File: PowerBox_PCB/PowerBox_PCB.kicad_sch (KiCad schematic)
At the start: 24 parts, among them SW1 SW_DPDT_x2

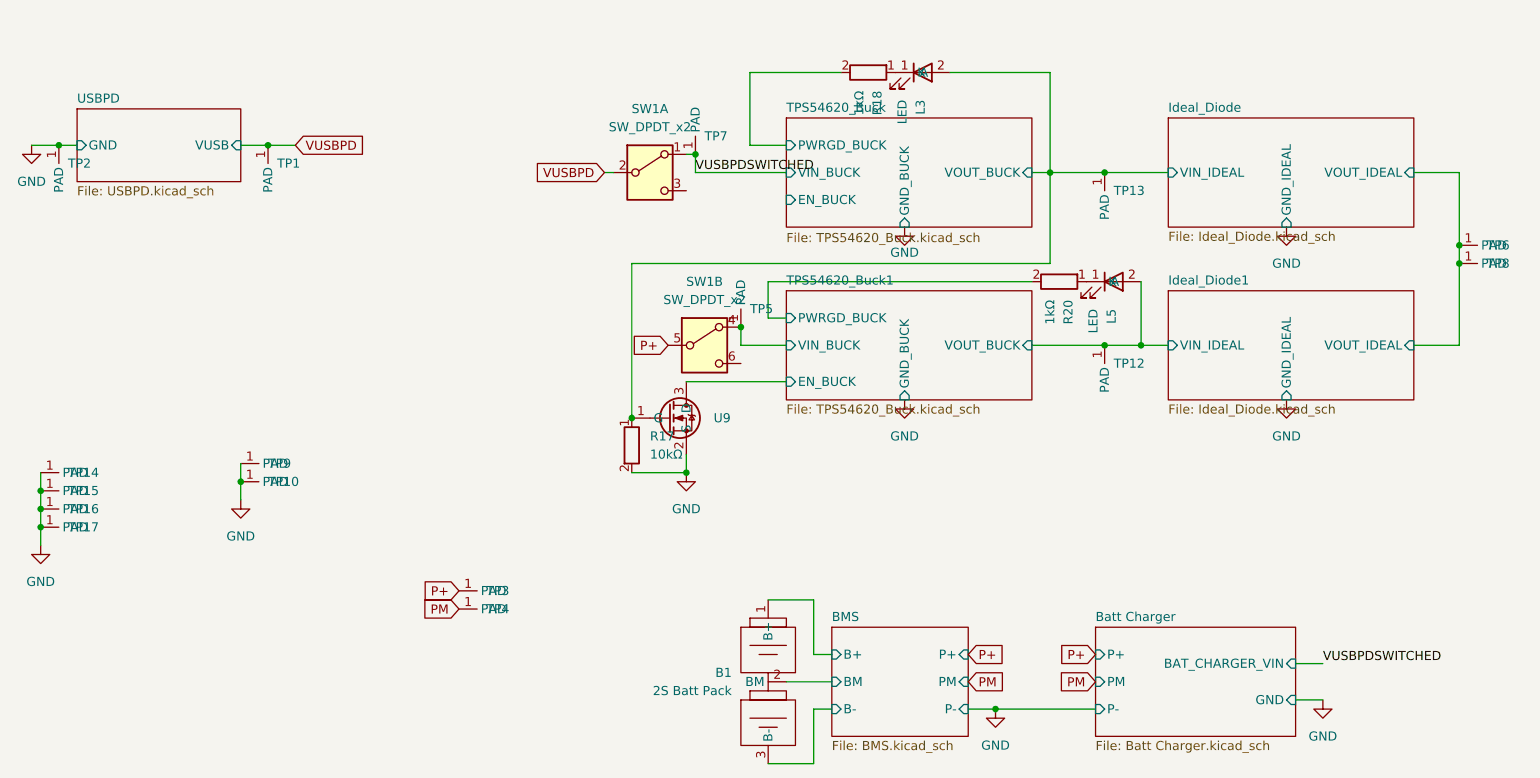
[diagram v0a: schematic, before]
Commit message: .
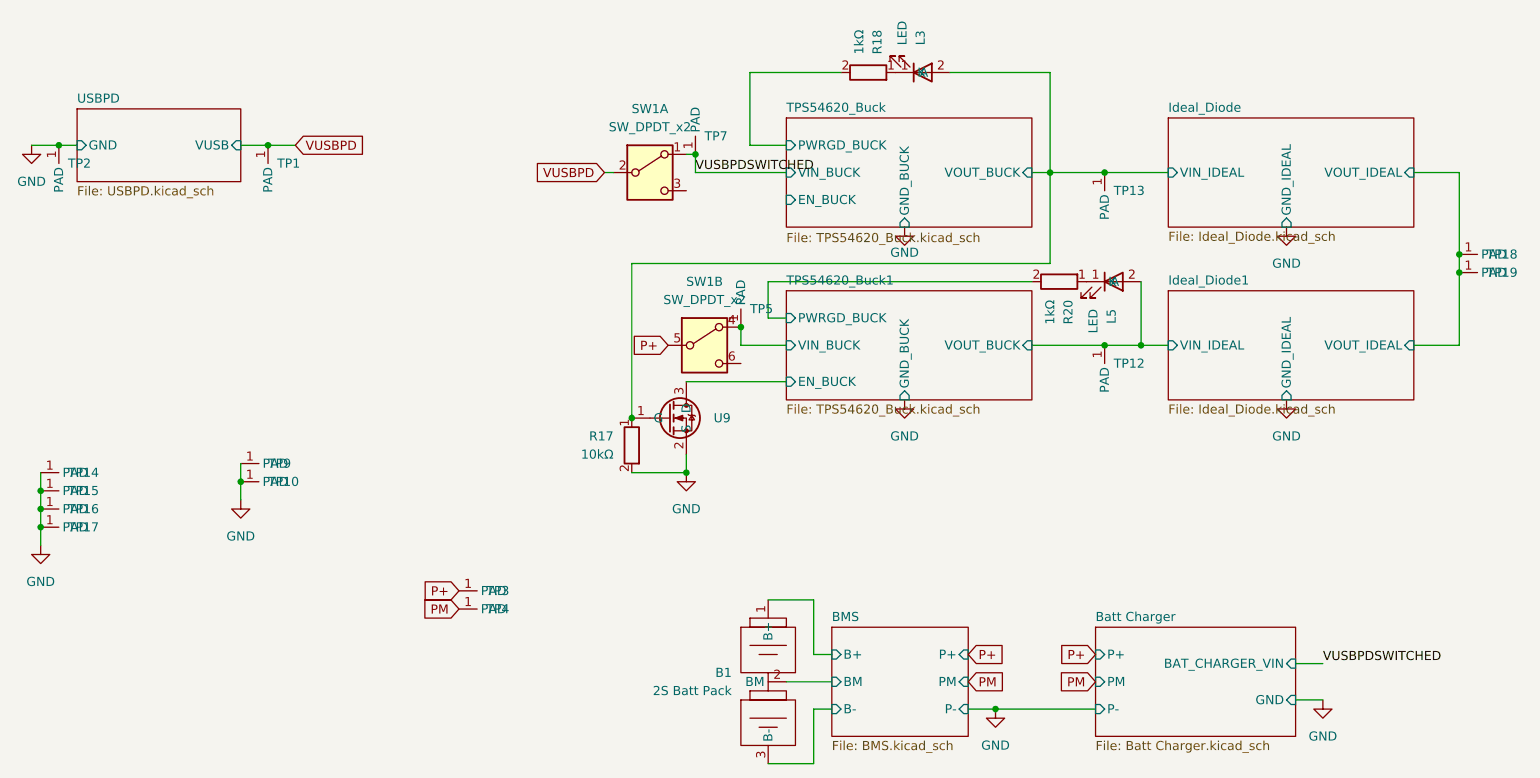
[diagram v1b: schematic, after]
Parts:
- removed TP6, TP8: (no value), Custom_Footprints:PAD-2x2, symbol Custom_Symbols:Pad-2x2
- added TP18, TP19: (no value), Custom_Footprints:PAD-2x2-ThroughHole, symbol Custom_Symbols:Pad-2x2-ThroughHole
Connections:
- net Ideal_Diode/VOUT_IDEAL: now also TP18.1 (PAD), TP19.1 (PAD)

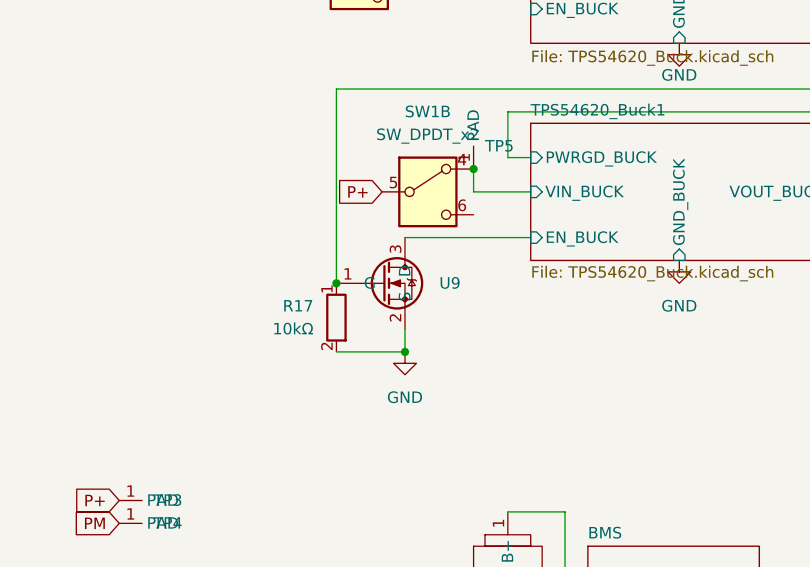
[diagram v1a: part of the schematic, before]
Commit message: fix bom
bom
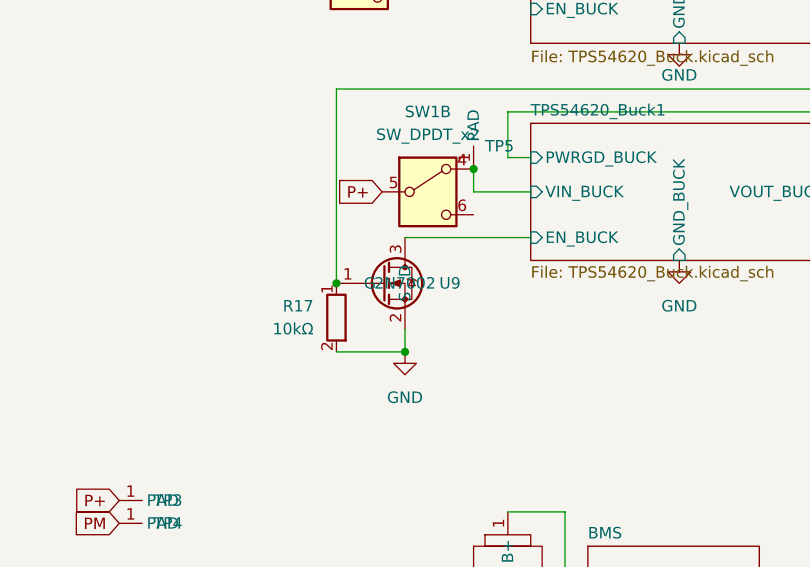
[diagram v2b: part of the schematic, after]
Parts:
- U9: value (none) -> 2N7002
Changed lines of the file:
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@@
 			)
 		)
-		(property "Value" ""
+		(property "Value" "2N7002"
 			(at 127 81.28 0)
 			(show_name no)
